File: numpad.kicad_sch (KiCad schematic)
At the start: 59 parts, among them SW2 SW_Push, U1 BlackPill_STLINK, U4 TRRS

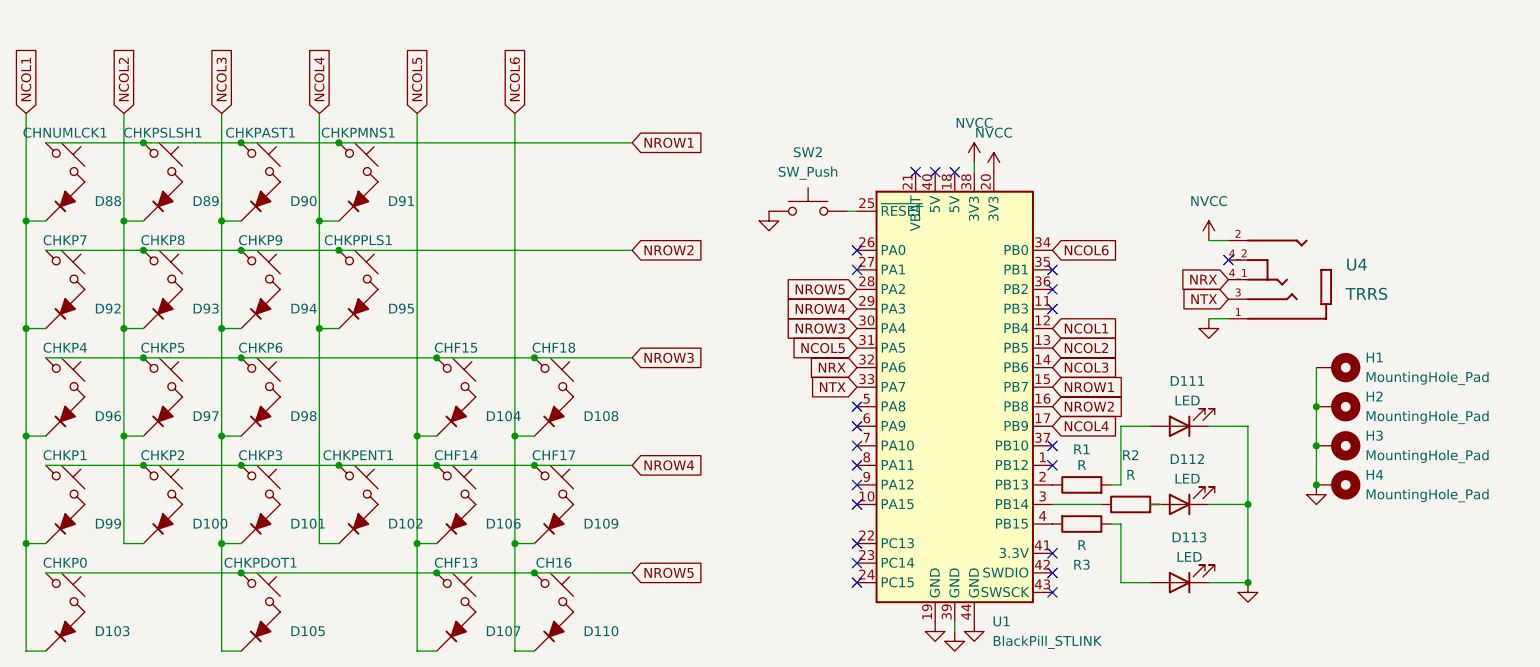
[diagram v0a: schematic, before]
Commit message: PDF Exports
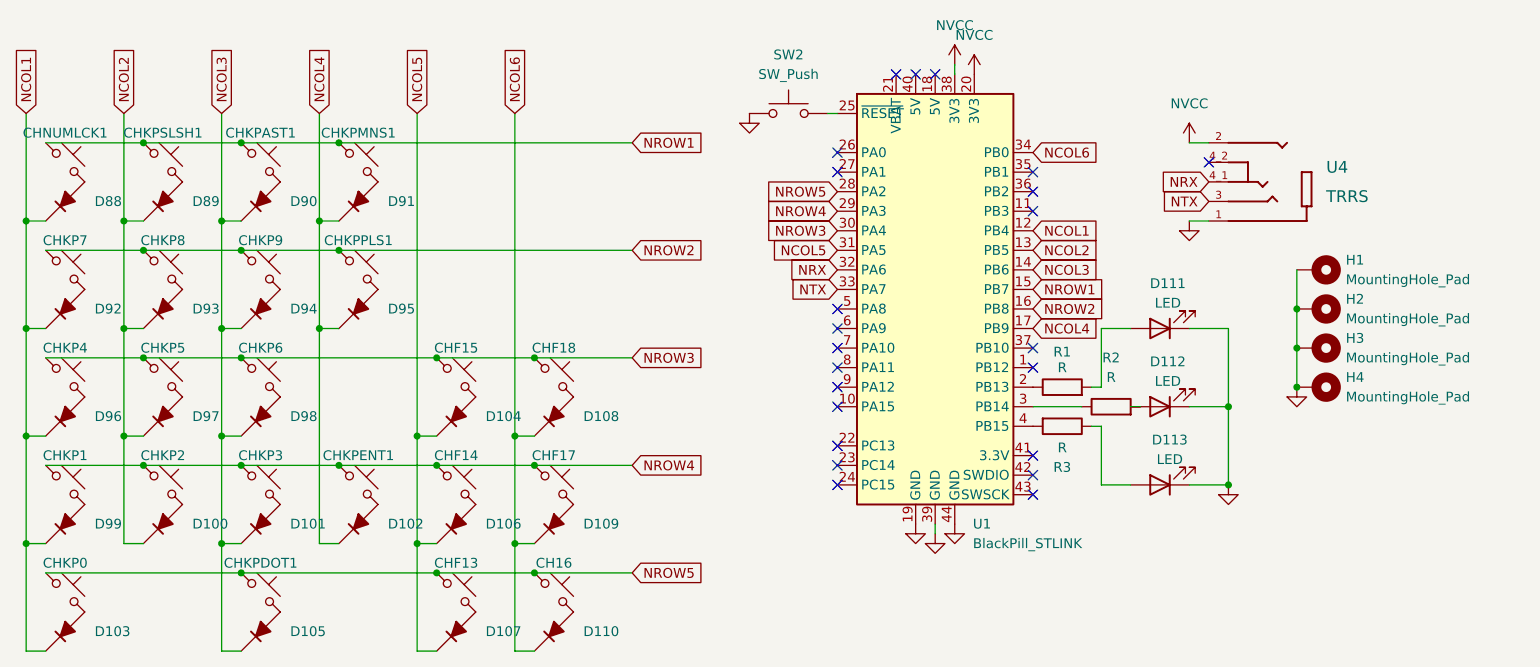
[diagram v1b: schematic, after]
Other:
- moved on the sheet: D111, D112, D113, H1, H2, H3, H4, R1, R2, R3, SW2, U1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
